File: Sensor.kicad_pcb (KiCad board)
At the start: 2 copper layers, 13 parts, among them J1 ProgPins, J2 Barrel, U10 ATtiny1616-S, U2 LDO, U9 MCP9700Ax-ELT

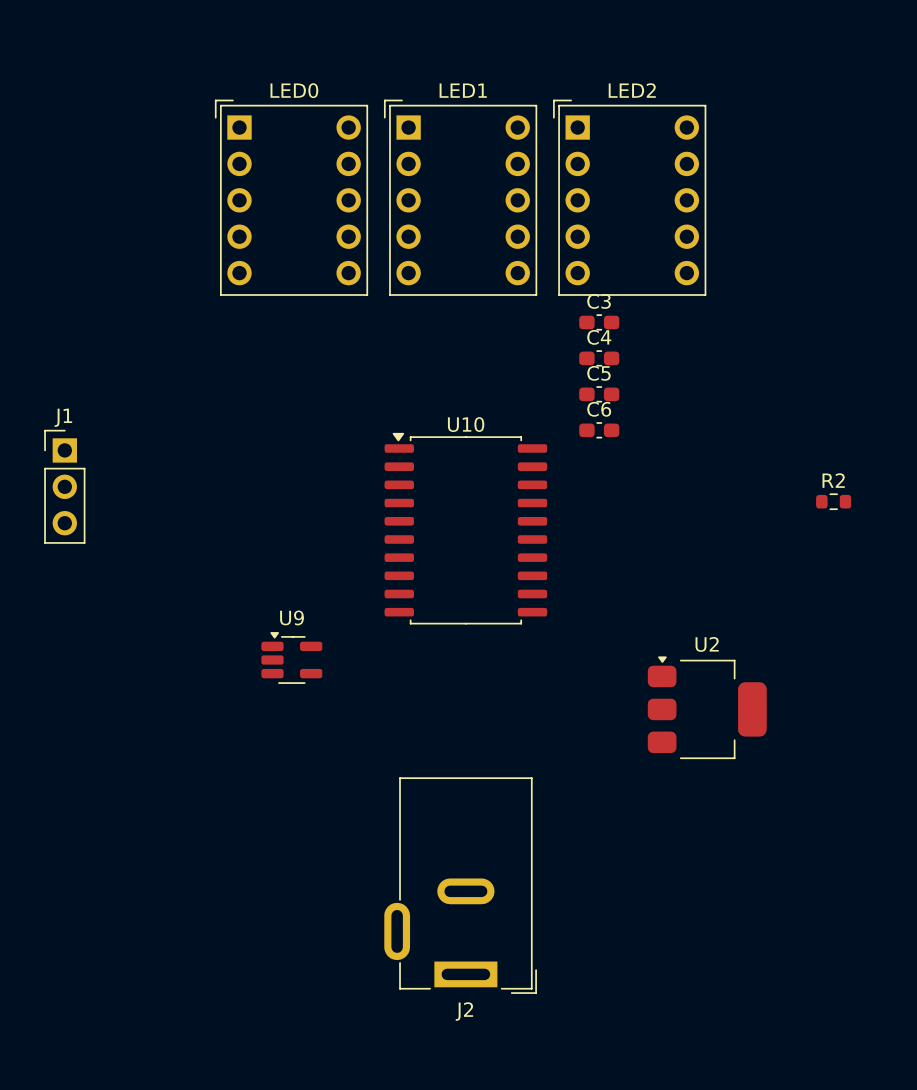
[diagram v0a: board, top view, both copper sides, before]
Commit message: feat: finished pcb
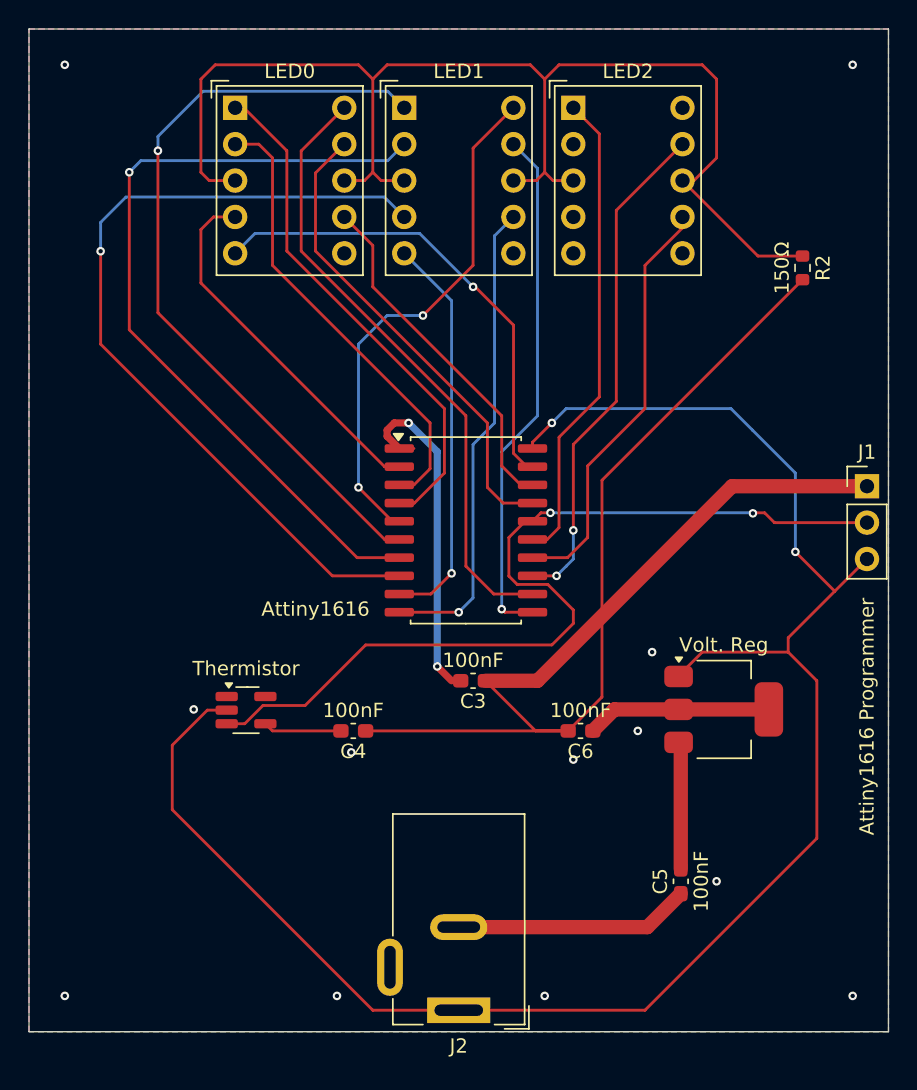
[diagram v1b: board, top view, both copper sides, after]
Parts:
- J1: value ProgPins -> Attiny1616 Programmer
- R2: value 150 Ohms -> 150Ω
- Volt. Reg: renamed from U2
- moved J1 56.1 mm to (169.5, 112.9)
- moved C5 34.5 mm to (156.5, 140.5), turned to 90 degrees
- moved C4 31.2 mm to (133.6, 130.0), turned to 180 degrees
- moved C3 26.5 mm to (142.0, 126.5), turned to 180 degrees
- moved C6 21.0 mm to (149.5, 130.0), turned to 180 degrees
- moved R2 16.5 mm to (165.0, 97.7), turned to -90 degrees
- moved Thermistor 4.74 mm to (126.2, 128.6)
- moved J2 2.55 mm to (141.0, 149.5)
- moved LED1 1.41 mm to (137.2, 86.5)
- moved LED2 1.41 mm to (149.0, 86.5)
- moved LED0 1.41 mm to (125.4, 86.5)
- moved Volt. Reg 1.15 mm to (159.5, 128.5)
- renumbered U10 to Attiny1616, U9 to Thermistor
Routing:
- net GND: track 0.00 -> 127.1 mm, vias 0 -> 14
- net /5V: track 0.00 -> 91.9 mm
- net Net-(LED0-CA-Pad3): track 0.00 -> 89.0 mm
- net Net-(J1-Pin_2): track 0.00 -> 62.2 mm, vias 0 -> 2
- net /SEG1-E: track 0.00 -> 58.6 mm, vias 0 -> 1
- net /SEG1-F: track 0.00 -> 56.4 mm, vias 0 -> 1
- net /SEG1-G: track 0.00 -> 54.7 mm, vias 0 -> 1
- net /SEG0-A: track 0.00 -> 43.5 mm
- net /SEG1-B: track 0.00 -> 36.4 mm, vias 0 -> 1
- net /SEG1-A: track 0.00 -> 36.3 mm, vias 0 -> 2
- net /SEG0-G: track 0.00 -> 35.9 mm
- net /SEG2-B: track 0.00 -> 35.5 mm, vias 0 -> 2
- net /SEG2-G: track 0.00 -> 33.4 mm
- net /SEG0-B: track 0.00 -> 33.4 mm
- net /SEG1-C: track 0.00 -> 33.3 mm, vias 0 -> 1
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- added copper zone on B.Cu, net GND
- added copper zone on F.Cu, net GND
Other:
- board outline added: 60 x 70 mm
